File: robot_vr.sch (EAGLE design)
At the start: 35 parts, among them CN10 SSM-119-L-DV, CN7 SSM-119-L-DV

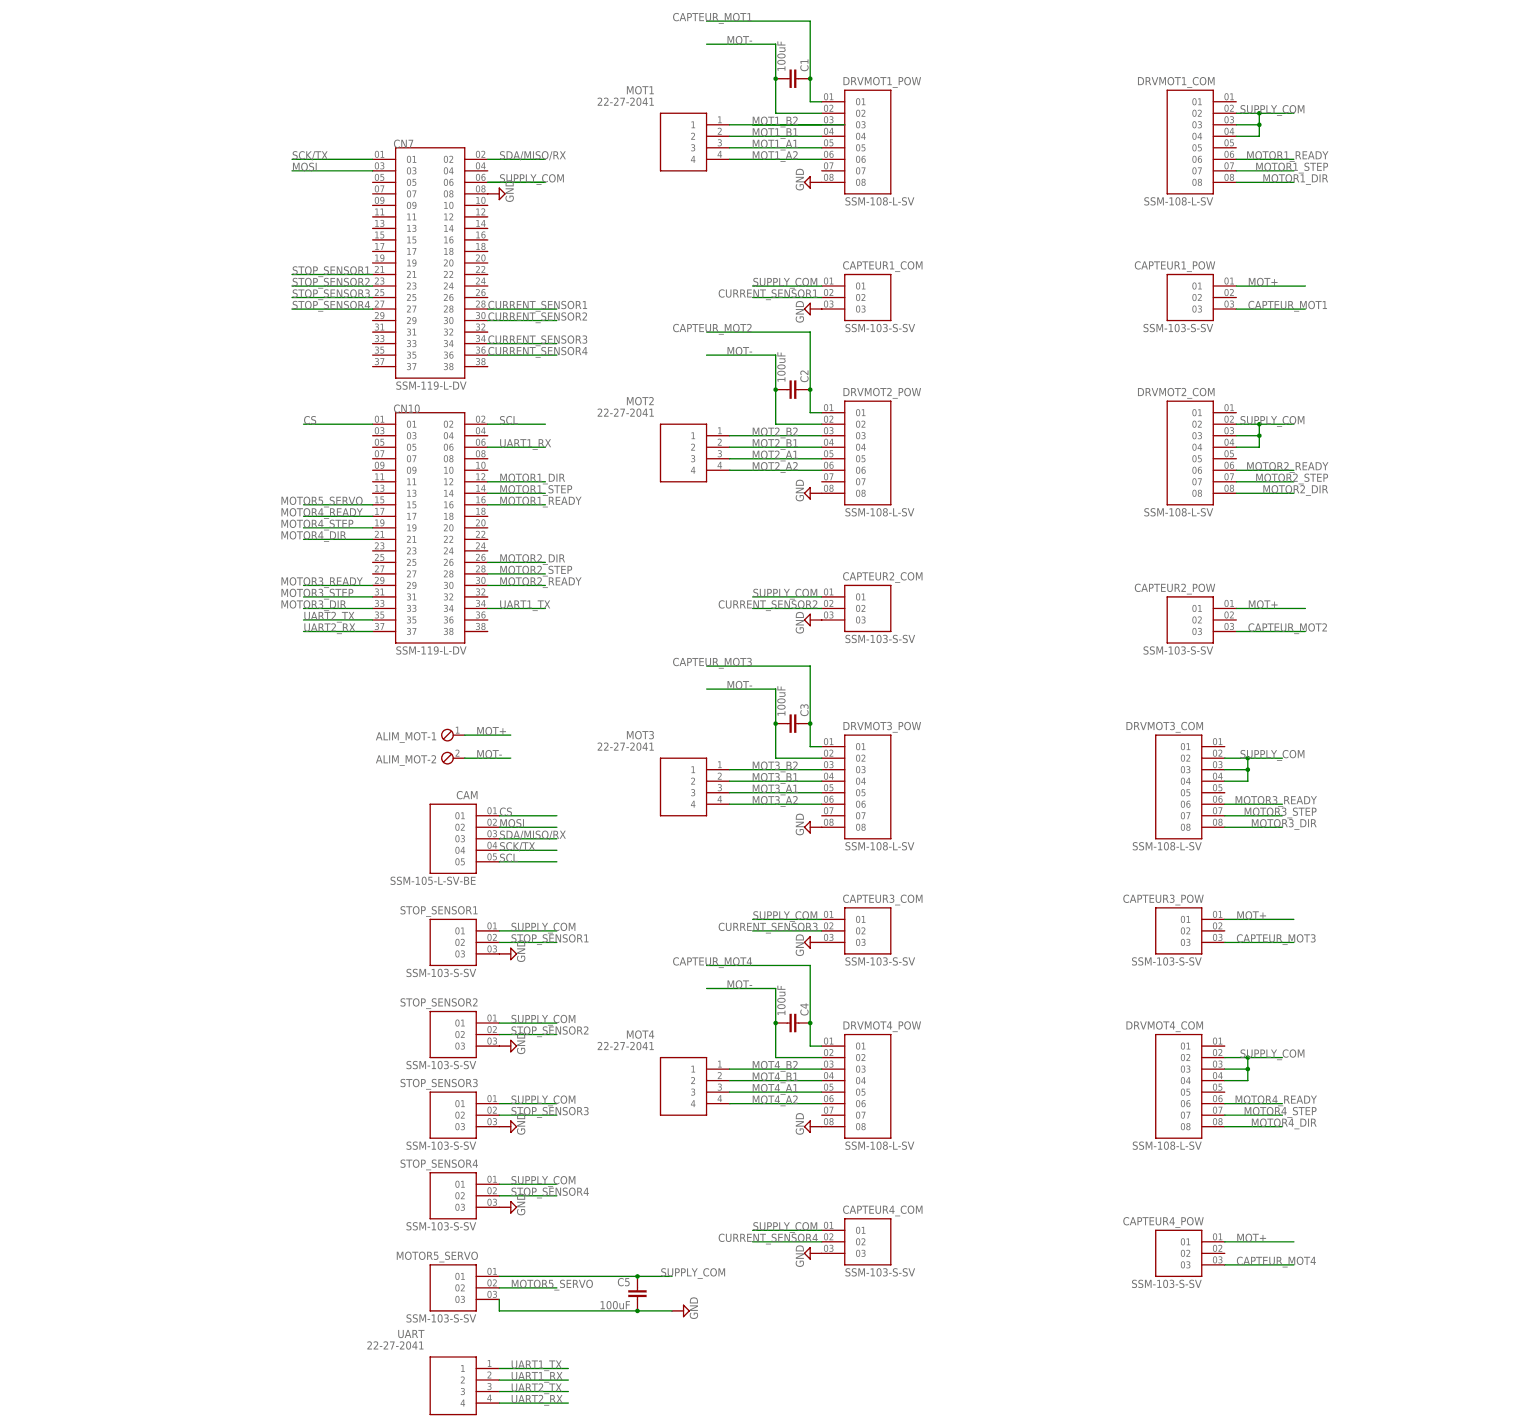
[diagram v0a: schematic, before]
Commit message: Add files via upload
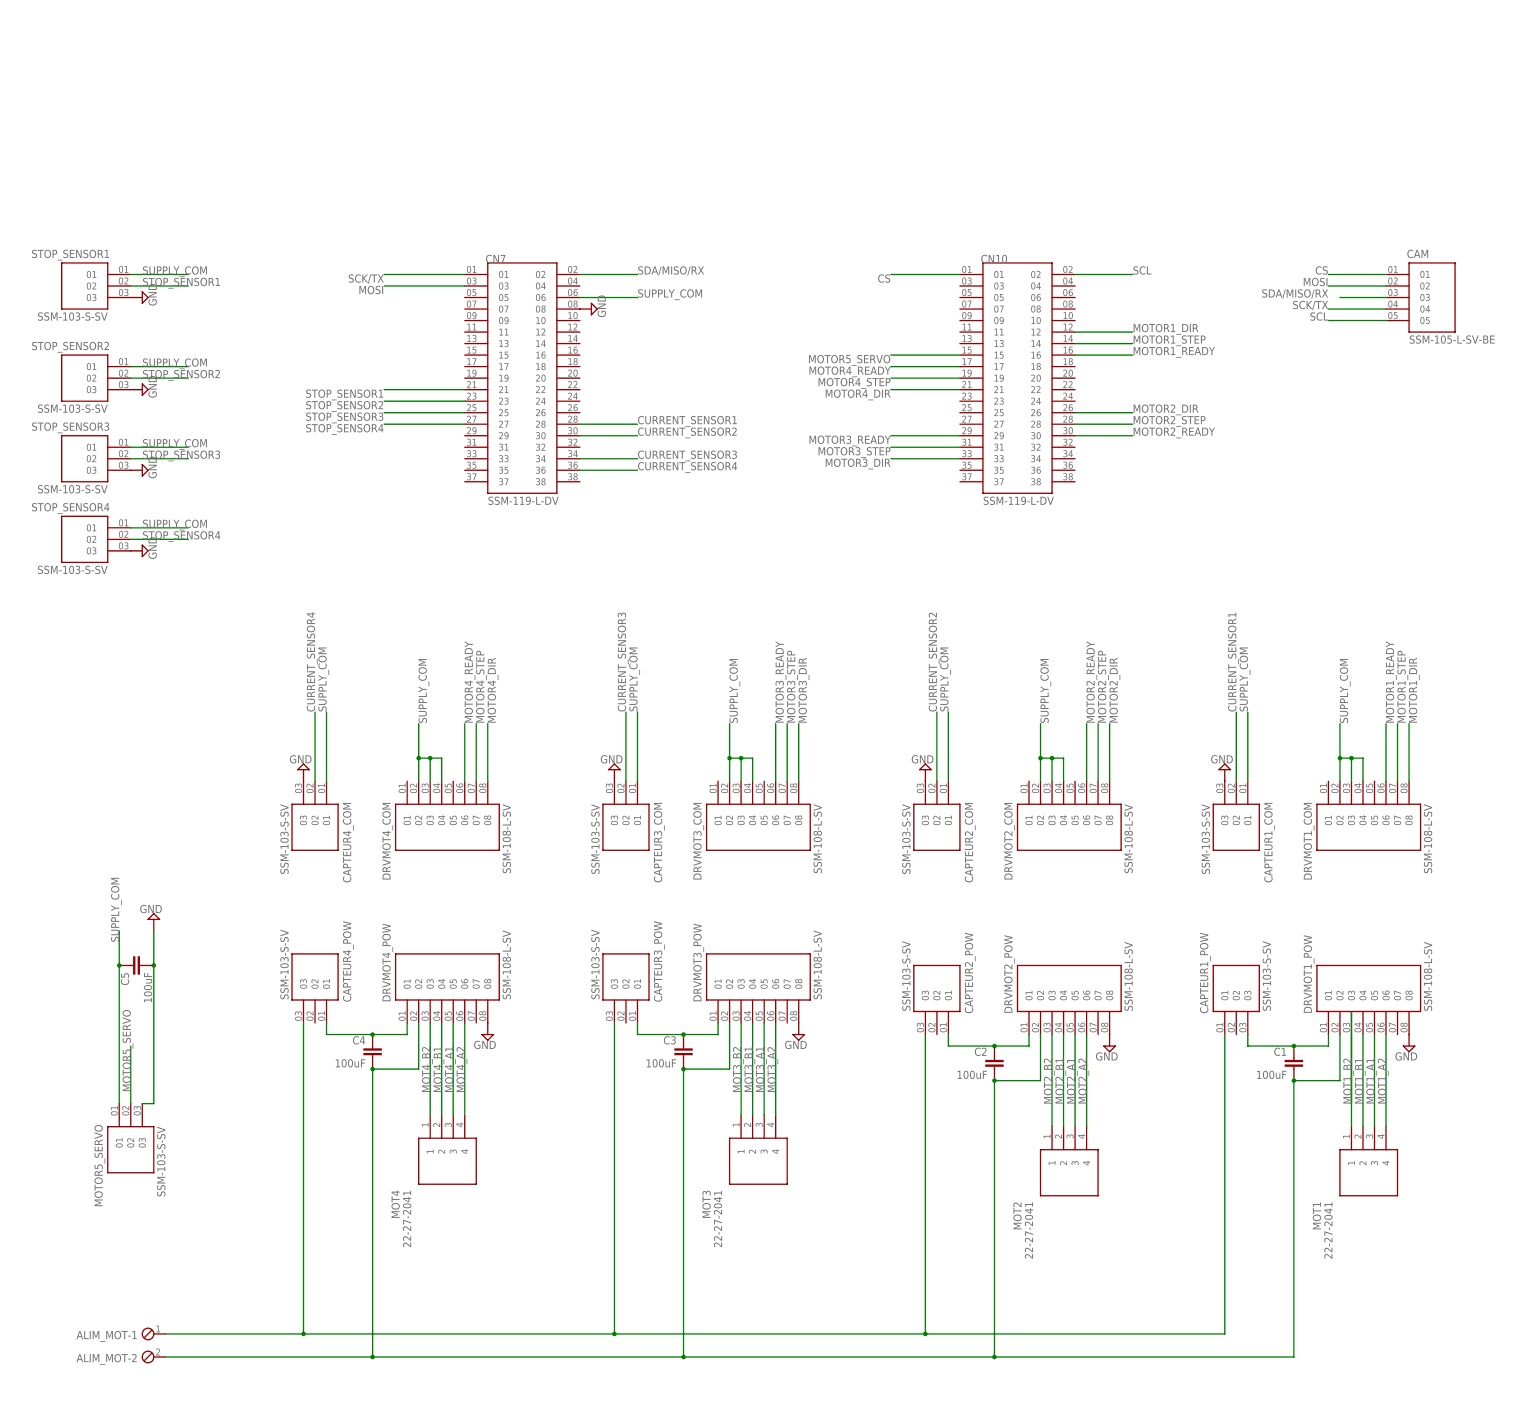
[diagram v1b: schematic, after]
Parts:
- removed UART: 22-27-2041, 22-27-2041:22-27-2041
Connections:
- removed net MOT+: ALIM_MOT-1.1, CAPTEUR1_POW.01, CAPTEUR2_POW.01, CAPTEUR3_POW.01, CAPTEUR4_POW.01
- removed net UART1_RX: CN10.06, UART.2
- removed net UART1_TX: CN10.34, UART.1
- removed net UART2_RX: CN10.37, UART.4
- removed net UART2_TX: CN10.35, UART.3
- new net N$1: ALIM_MOT-1.1, CAPTEUR1_POW.01, CAPTEUR2_POW.03, CAPTEUR3_POW.03, CAPTEUR4_POW.03
- net CAPTEUR_MOT2: now also CAPTEUR2_POW.01; no longer CAPTEUR2_POW.03
- net CAPTEUR_MOT3: now also CAPTEUR3_POW.01; no longer CAPTEUR3_POW.03
- net CAPTEUR_MOT4: now also CAPTEUR4_POW.01; no longer CAPTEUR4_POW.03
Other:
- moved on the sheet: ALIM_MOT-1, ALIM_MOT-2, C1, C2, C3, C4, C5, CAM, CAPTEUR1_COM, CAPTEUR1_POW, CAPTEUR2_COM, CAPTEUR2_POW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
